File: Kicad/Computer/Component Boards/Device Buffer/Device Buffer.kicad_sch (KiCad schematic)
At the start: 18 parts, among them IC1 SN74ABT245BDBR, IC2 SN74ABT245BDBR, IC3 SN74ABT245BDBR, IC4 SN74ABT245BDBR, IC5 AP7365-33WG-7, J2 Conn_02x32_Counter_Clockwise

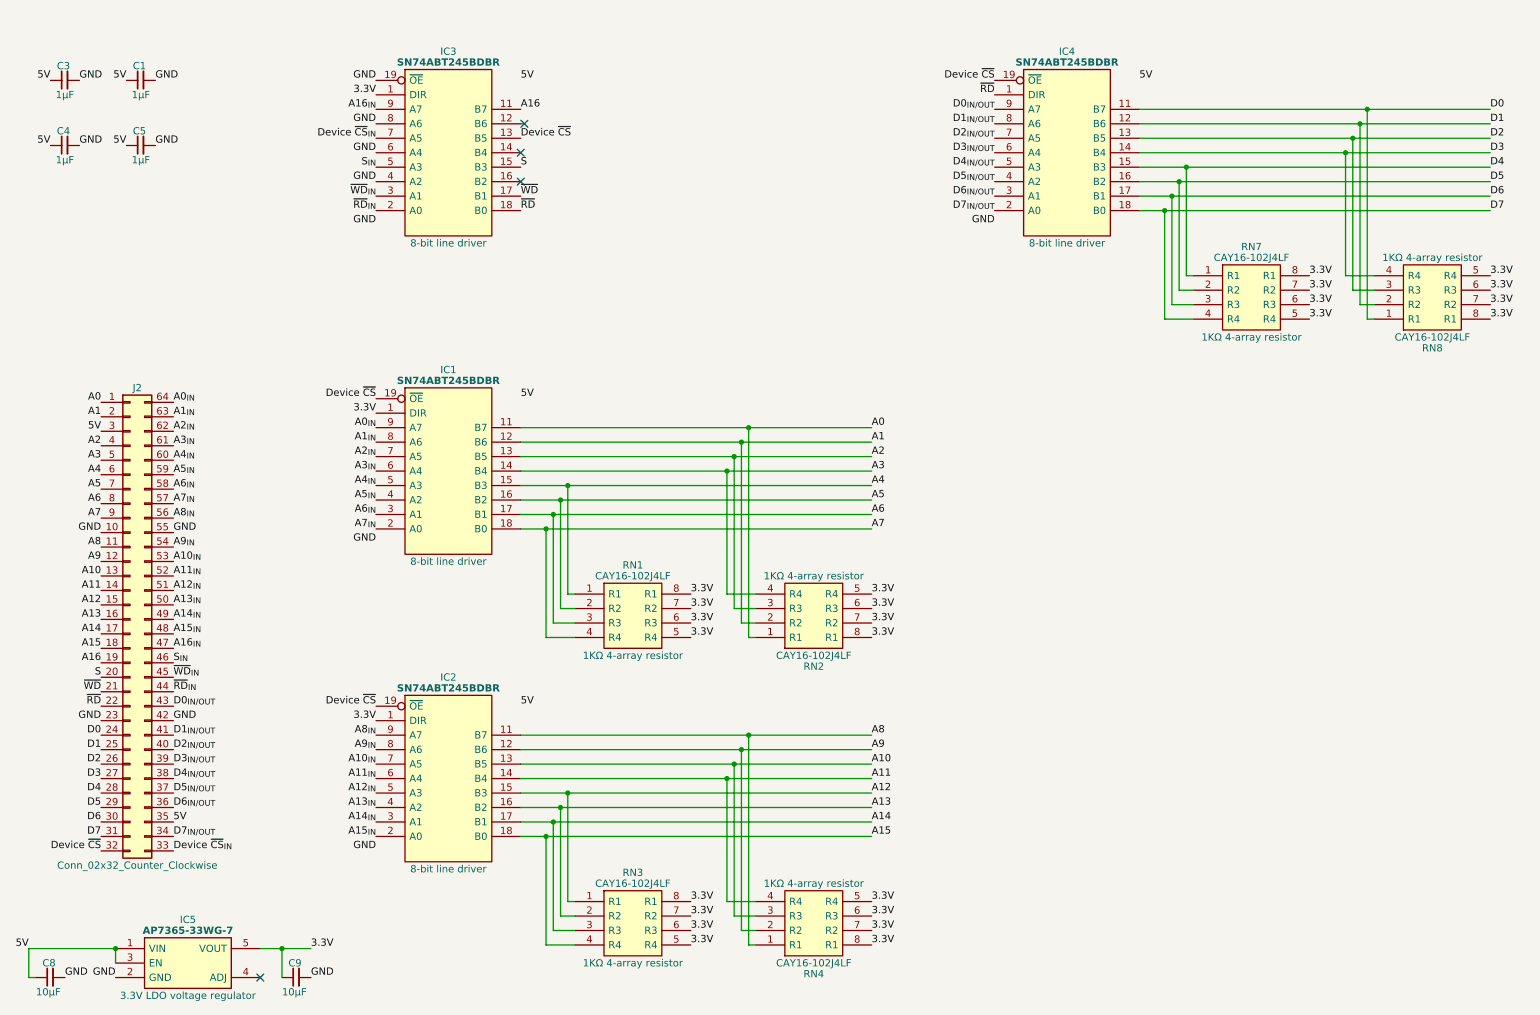
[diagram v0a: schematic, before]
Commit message: Generating more Gerbers.
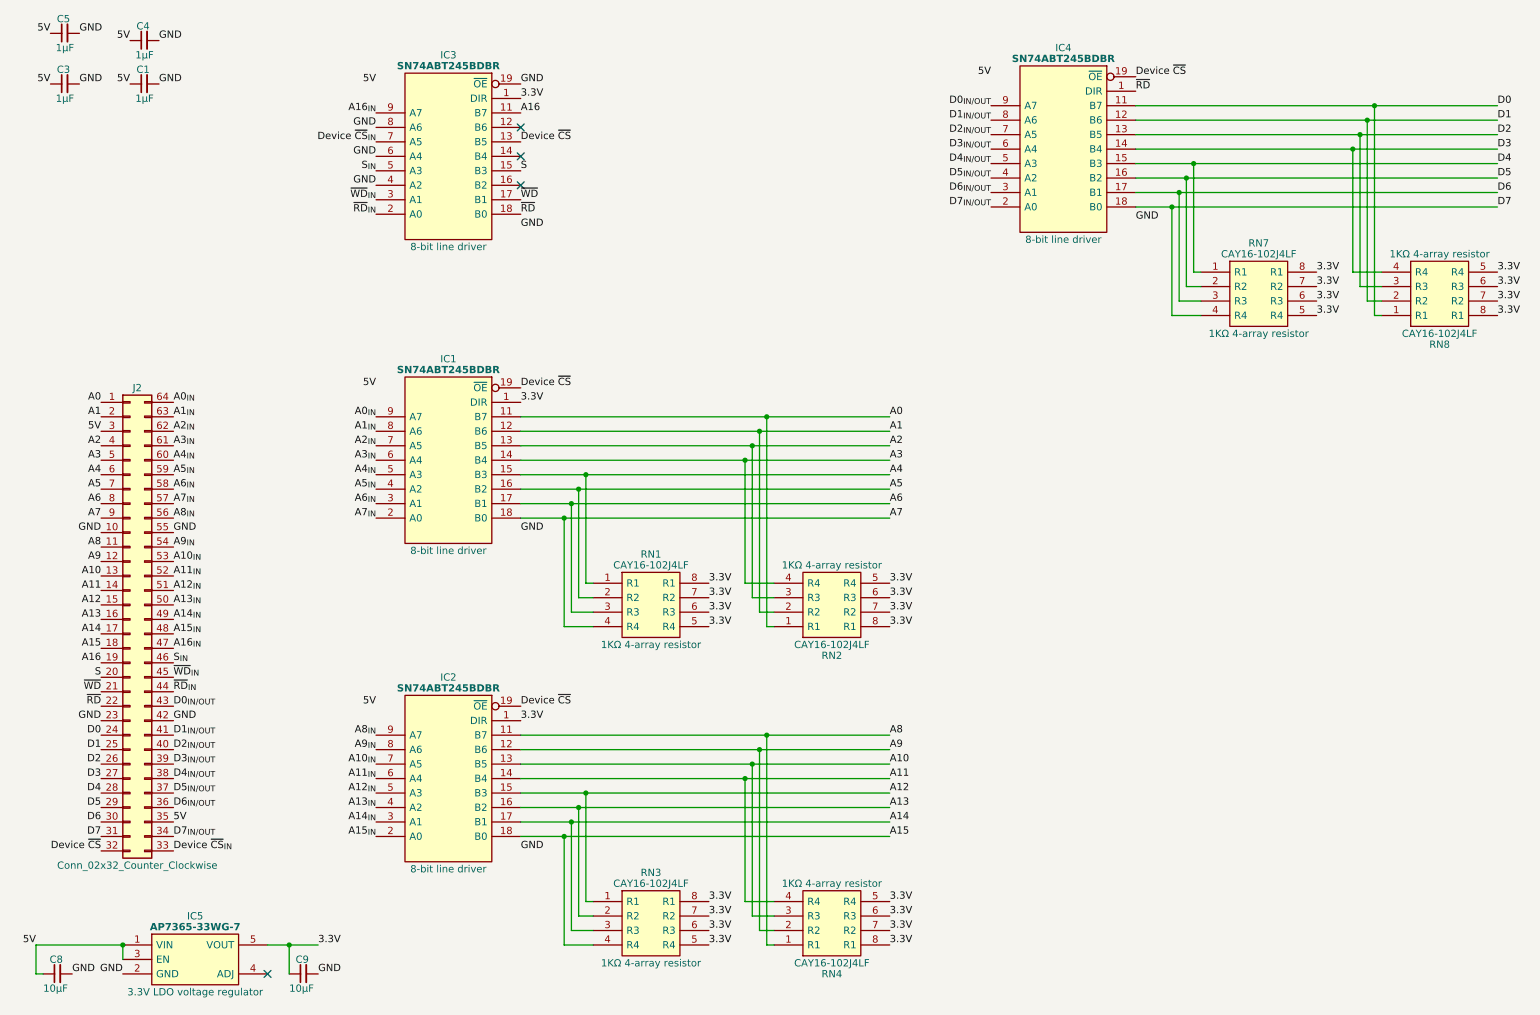
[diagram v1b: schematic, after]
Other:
- moved on the sheet: C1, C3, C4, C5, C8, C9, IC1, IC3, IC4, IC5, RN1, RN2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
